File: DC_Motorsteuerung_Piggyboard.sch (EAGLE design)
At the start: 16 parts, among them X1 PFVERB10

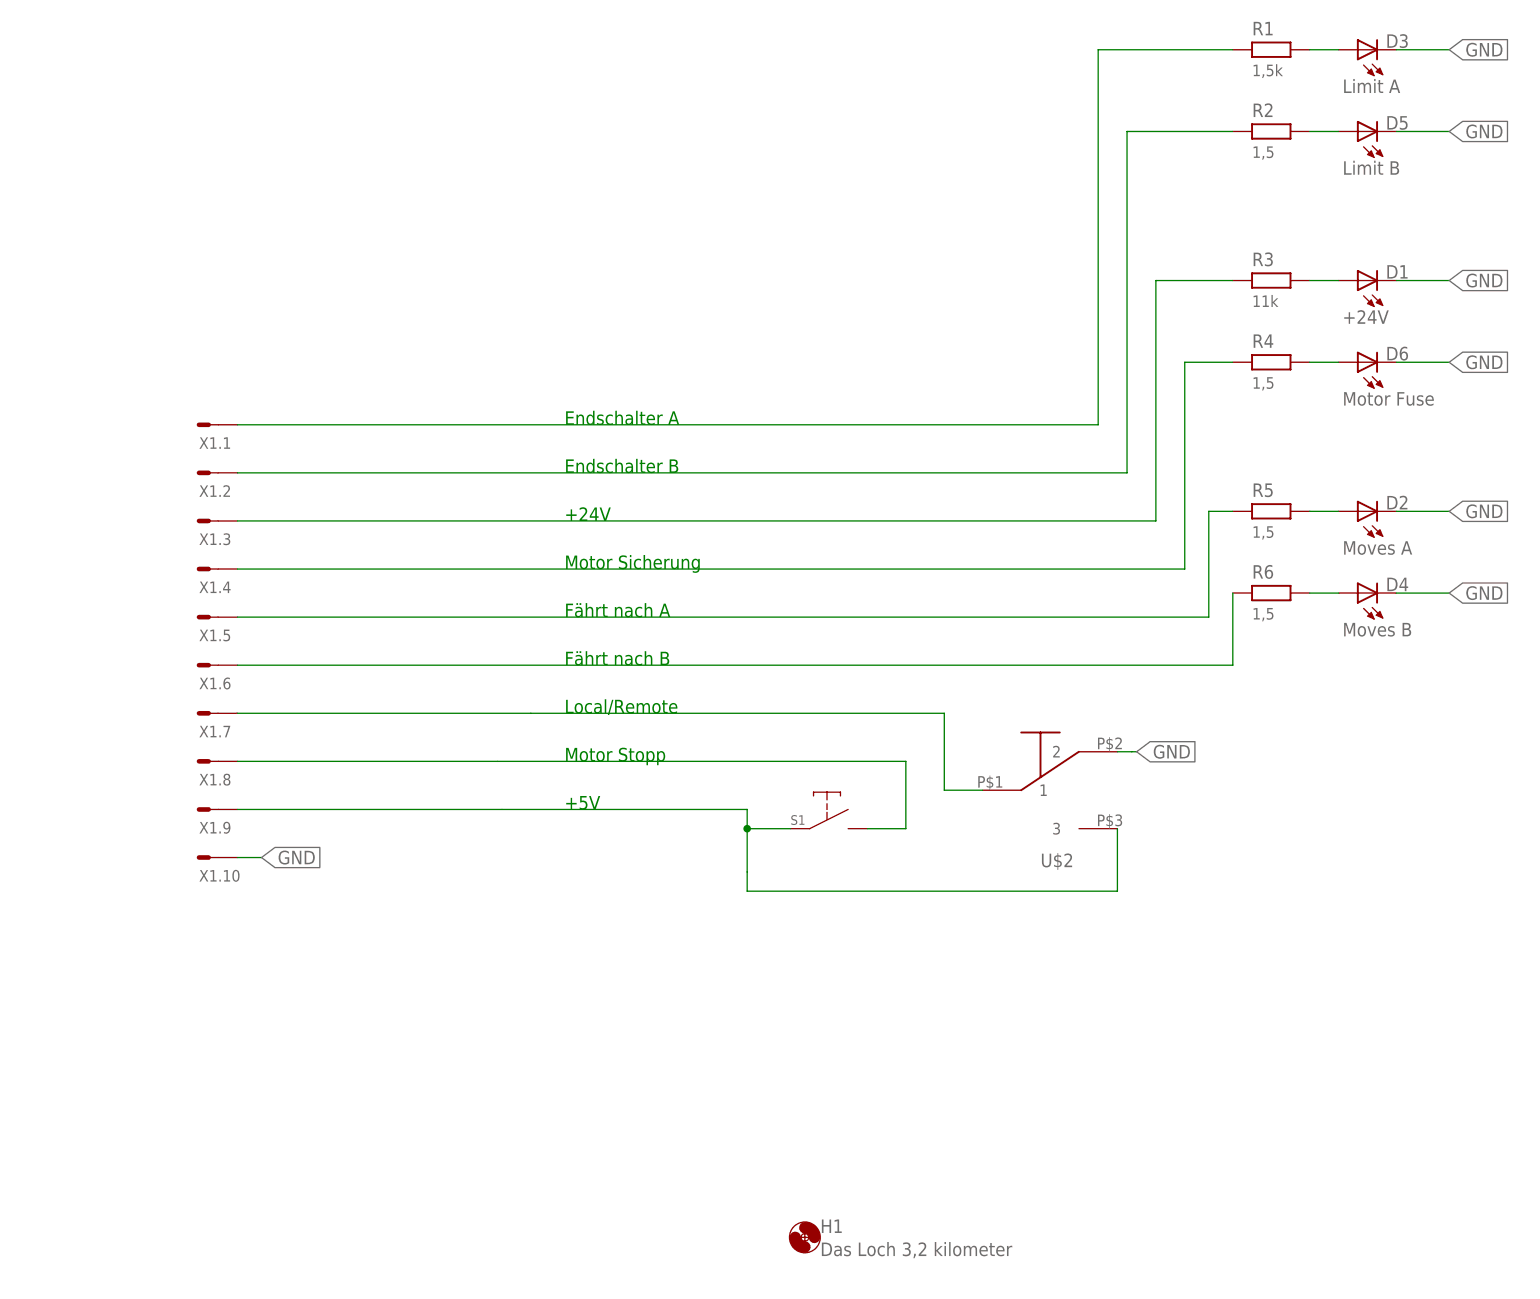
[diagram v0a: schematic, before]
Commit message: Piggyboard updated and finished !! (RGB-LED included)
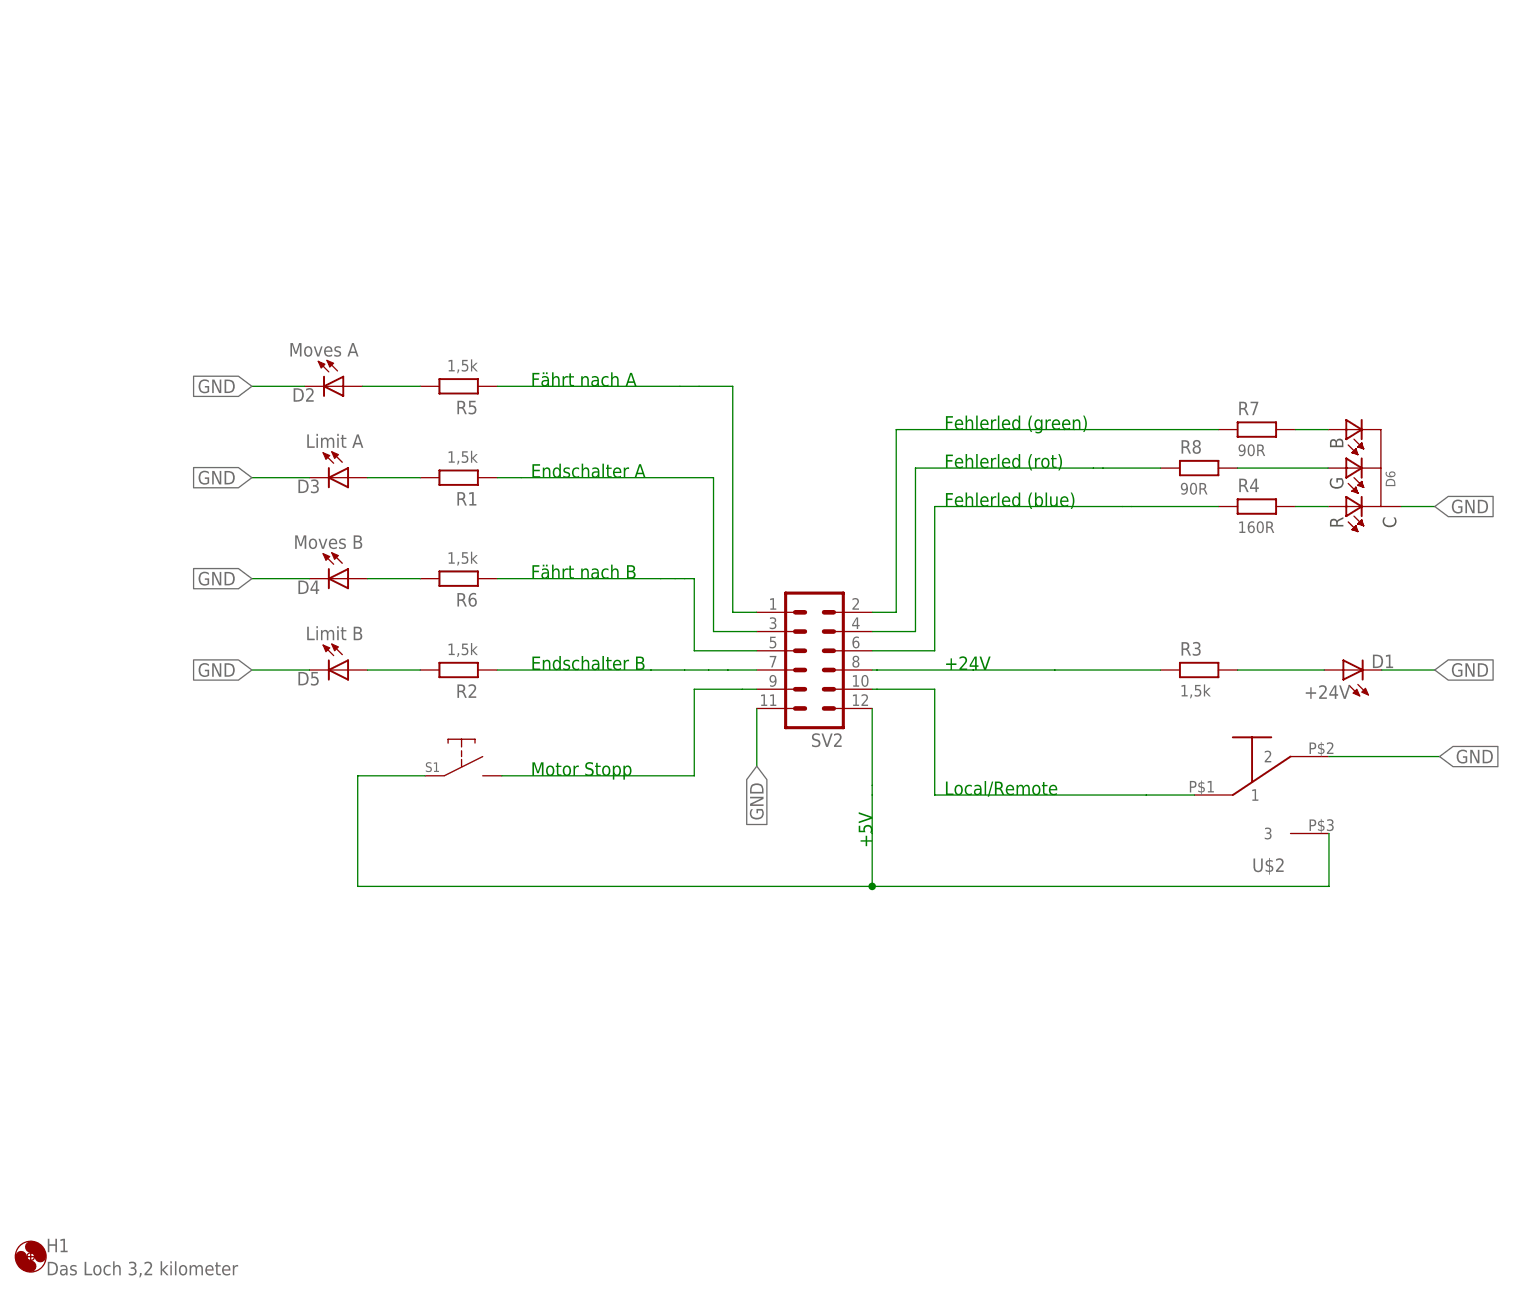
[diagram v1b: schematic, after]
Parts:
- removed X1: PFVERB10, Connector:PFVERB10
- added R7, R8: 90R, Resistor:R_0,4W
- added SV2: (no value), con-lstb:MA06-2
- D6: value Motor Fuse -> (none); device Test:LED3MM -> LED:RGB_LED_5MM
- R2, R5, R6: value 1,5 -> 1,5k
- R3: value 11k -> 1,5k
- R4: value 1,5 -> 160R
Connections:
- removed net N$8: S1.C, U$2.3, X1.9.1
- new net N$16: R4.1, SV2.6
- new net N$17: D6.BLUE, R7.2
- new net N$18: D6.GREEN, R8.2
- new net N$19: D6.RED, R4.2
- new net N$20: R6.1, SV2.5
- net GND: now also D6.CATHODE, SV2.11; no longer D6.C, X1.10.1
- net N$1: now also SV2.7; no longer X1.2.1
- net N$11: now also S1.C, SV2.12, U$2.3; no longer R6.1, X1.6.1
- net N$12: now also SV2.1; no longer X1.5.1
- net N$15: now also R7.1, SV2.2; no longer D6.A, R4.2
- net N$3: now also SV2.3; no longer X1.1.1
- net N$5: now also R8.1, SV2.4; no longer R4.1, X1.4.1
- net N$6: now also SV2.8; no longer X1.3.1
- net N$7: now also SV2.9; no longer X1.8.1
- net N$9: now also SV2.10; no longer X1.7.1
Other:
- note added: "Fehlerled (blue)"
- note added: "Fehlerled (green)"
- note added: "Fehlerled (rot)"
- note removed: "Motor Sicherung"
- moved on the sheet: D1, D2, D3, D4, D5, H1, R1, R2, R3, R4, R5, R6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
